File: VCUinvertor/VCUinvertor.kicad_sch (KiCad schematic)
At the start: 100 parts, among them J1 NXP1, J2 Conn_02x10_Odd_Even, J3 NXP2, J4 Conn_02x10_Odd_Even, J5 Conn_02x10_Odd_Even, J6 Conn_02x10_Odd_Even, J7 PowerSupply, J8 CAN_NXP, J9 BACKLIGHT, Q1 BSS138, Q10 BSS138, Q2 BSS138, Q3 BSS138, Q4 BSS138, Q5 BSS138, Q6 BSS138, Q7 BSS138, Q8 BSS138, Q9 BSS138, U1 TJA1448ATK, U2 REF3433T, U3 TLV76150DCY

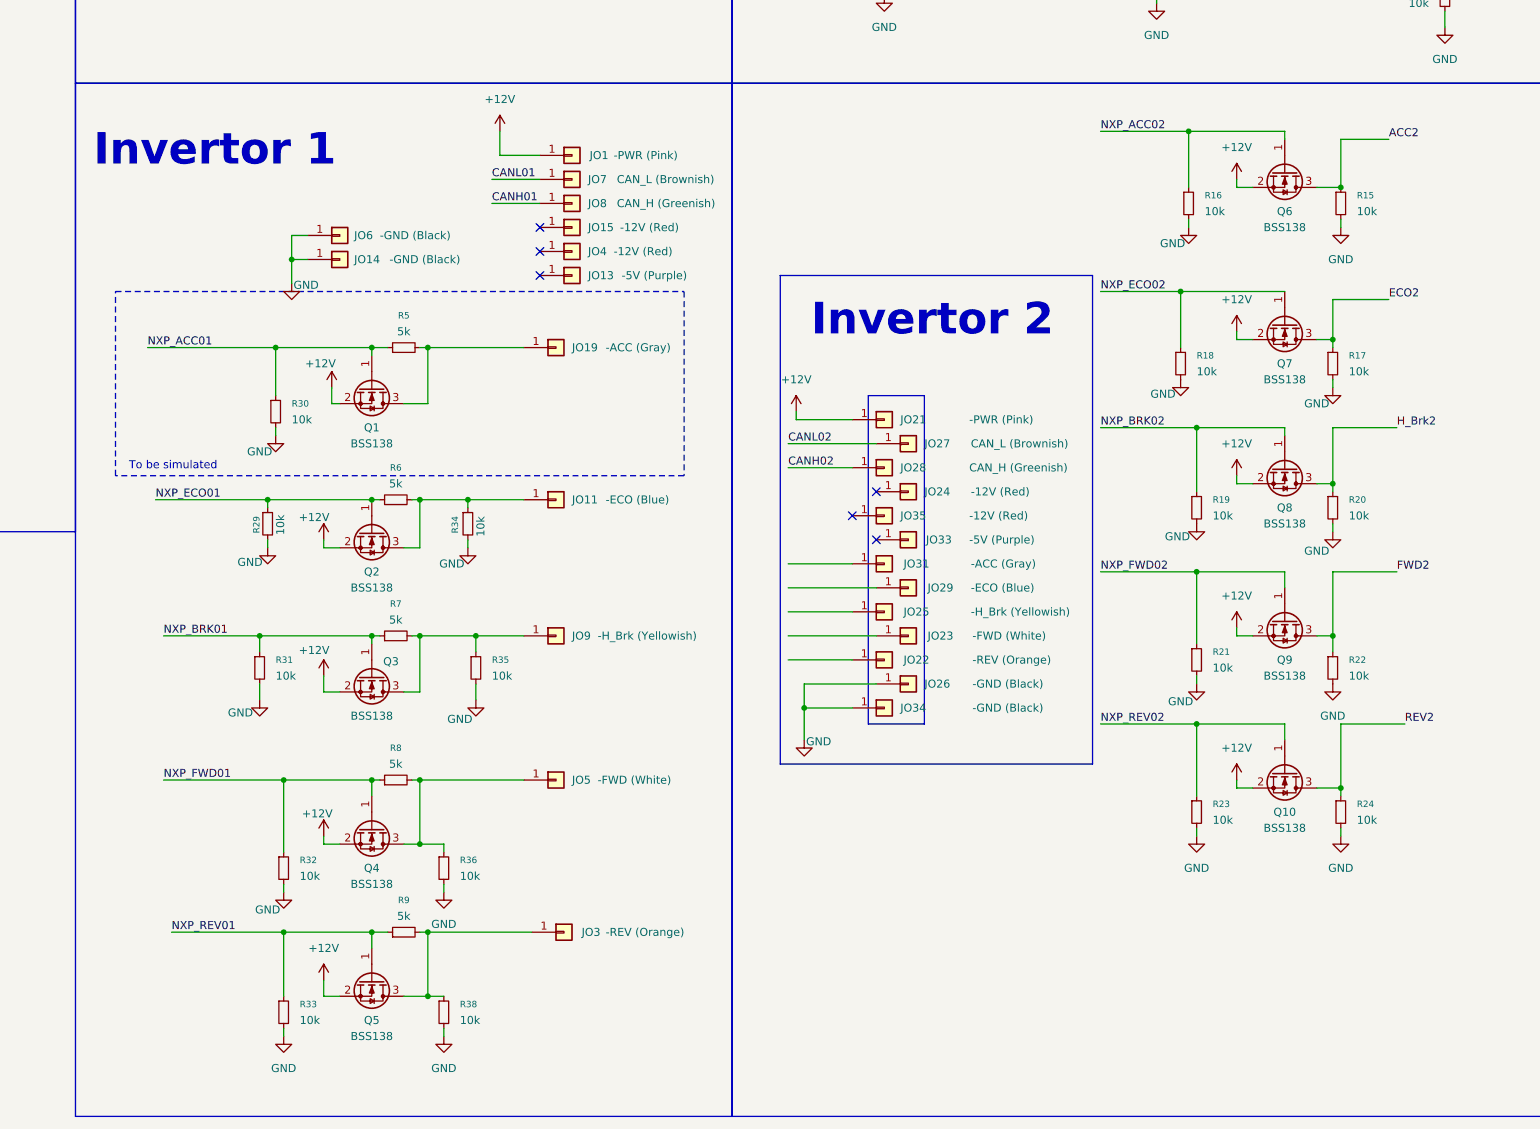
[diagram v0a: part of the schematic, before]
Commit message: NMOS_Simulation_Selection
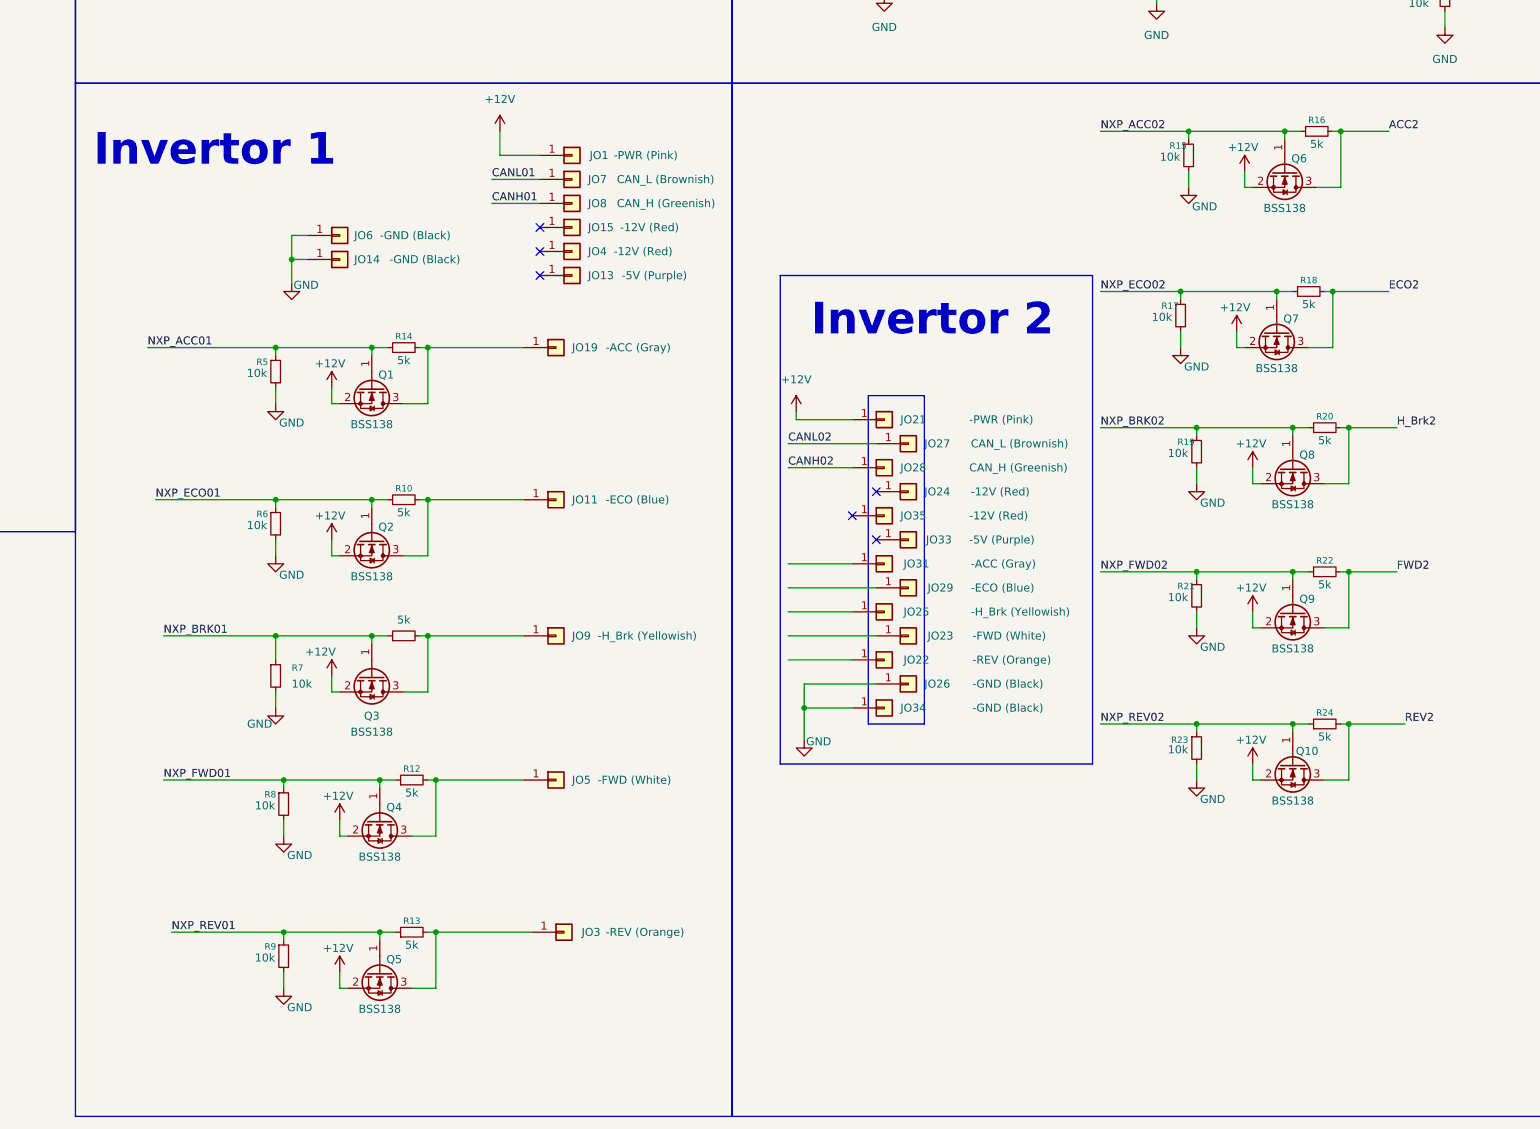
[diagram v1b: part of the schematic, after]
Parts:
- removed R29, R30, R31, R32, R33, R34, R35, R36, R38: 10k, symbol Device:R_Small
- added R10, R11, R12, R13, R14: 5k, symbol Device:R_Small
- R16, R18, R20, R22, R24: value 10k -> 5k
- R5, R6, R7, R8, R9: value 5k -> 10k
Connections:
- net ACC2: now also R16.2; no longer R15.1
- net ECO2: now also R18.2; no longer R17.1
- net FWD2: now also R22.2; no longer R22.1
- net GND: now also R5.2, R6.2, R7.2, R8.2, R9.2; no longer R16.2, R18.2, R20.2, R22.2, R24.2
- net H_Brk2: now also R20.2; no longer R20.1
- net NXP_ACC01: now also R14.1
- net NXP_ACC02: now also R15.1
- net NXP_BRK01: now also R11.1
- net NXP_BRK02: now also R20.1
- net NXP_ECO01: now also R10.1
- net NXP_ECO02: now also R17.1
- net NXP_FWD01: now also R12.1
- net NXP_FWD02: now also R22.1
- net NXP_REV01: now also R13.1
- net NXP_REV02: now also R24.1
- net REV2: now also R24.2; no longer R24.1
- net at JO19.1 (Pin_1), Q1.3 (D): now also R14.2; no longer R5.2
- net at JO3.1 (Pin_1), Q5.3 (D): now also R13.2; no longer R9.2
- net at JO11.1 (Pin_1), Q2.3 (D): now also R10.2; no longer R6.2
- net at JO5.1 (Pin_1), Q4.3 (D): now also R12.2; no longer R8.2
- net at JO9.1 (Pin_1), Q3.3 (D): now also R11.2; no longer R7.2
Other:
- note removed: "To be simulated"
